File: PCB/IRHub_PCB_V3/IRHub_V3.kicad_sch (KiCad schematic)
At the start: 85 parts, among them Q1 UMH3N, SW1 SW_Push, U1 DRV2605LDGS

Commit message: power pcb done
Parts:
- 5V1, TP9, T_D+1, T_D-1, T_D6, T_D7, T_GND1, T_RX1, T_TX1: footprint TestPoint:TestPoint_Pad_D2.0mm -> TestPoint:TestPoint_Pad_D1.0mm
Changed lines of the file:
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@@
 			)
 		)
-		(property "Footprint" "TestPoint:TestPoint_Pad_D2.0mm"
+		(property "Footprint" "TestPoint:TestPoint_Pad_D1.0mm"
 			(at 267.97 156.21 0)
 			(effects
@@
 			)
 		)
-		(property "Footprint" "TestPoint:TestPoint_Pad_D2.0mm"
+		(property "Footprint" "TestPoint:TestPoint_Pad_D1.0mm"
 			(at 267.97 130.81 0)
 			(effects
@@
 			)
 		)
-		(property "Footprint" "TestPoint:TestPoint_Pad_D2.0mm"
+		(property "Footprint" "TestPoint:TestPoint_Pad_D1.0mm"
 			(at 267.97 149.86 0)
 			(effects
@@
 			)
 		)
-		(property "Footprint" "TestPoint:TestPoint_Pad_D2.0mm"
+		(property "Footprint" "TestPoint:TestPoint_Pad_D1.0mm"
 			(at 267.97 128.27 0)
 			(effects
@@
 			)
 		)
-		(property "Footprint" "TestPoint:TestPoint_Pad_D2.0mm"
+		(property "Footprint" "TestPoint:TestPoint_Pad_D1.0mm"
 			(at 267.97 147.32 0)
 			(effects
@@
 			)
 		)
-		(property "Footprint" "TestPoint:TestPoint_Pad_D2.0mm"
+		(property "Footprint" "TestPoint:TestPoint_Pad_D1.0mm"
 			(at 267.97 166.37 0)
 			(effects
@@
 			)
 		)
-		(property "Footprint" "TestPoint:TestPoint_Pad_D2.0mm"
+		(property "Footprint" "TestPoint:TestPoint_Pad_D1.0mm"
 			(at 267.97 158.75 0)
 			(effects
@@
 			)
 		)
-		(property "Footprint" "TestPoint:TestPoint_Pad_D2.0mm"
+		(property "Footprint" "TestPoint:TestPoint_Pad_D1.0mm"
 			(at 267.97 137.16 0)
 			(effects
@@
 			)
 		)
-		(property "Footprint" "TestPoint:TestPoint_Pad_D2.0mm"
+		(property "Footprint" "TestPoint:TestPoint_Pad_D1.0mm"
 			(at 267.97 139.7 0)
 			(effects

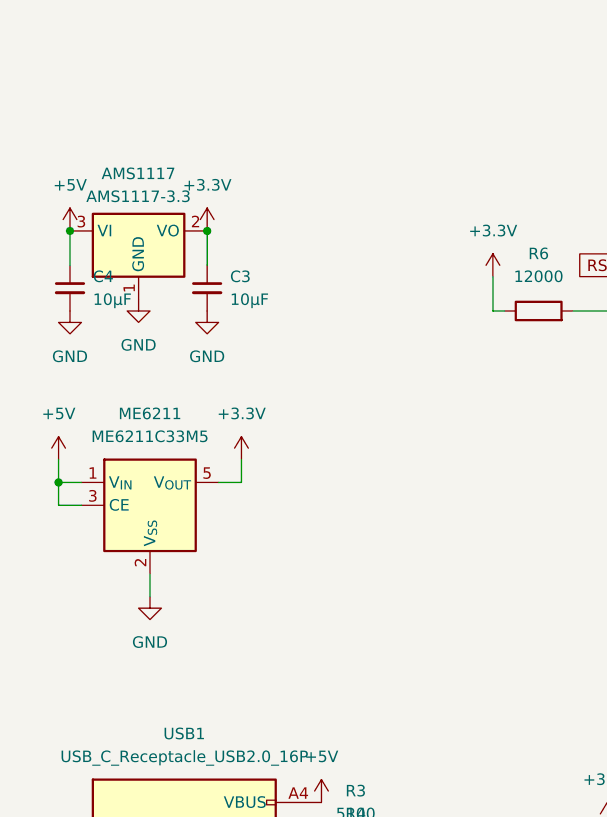
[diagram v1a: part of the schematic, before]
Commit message: finished placement
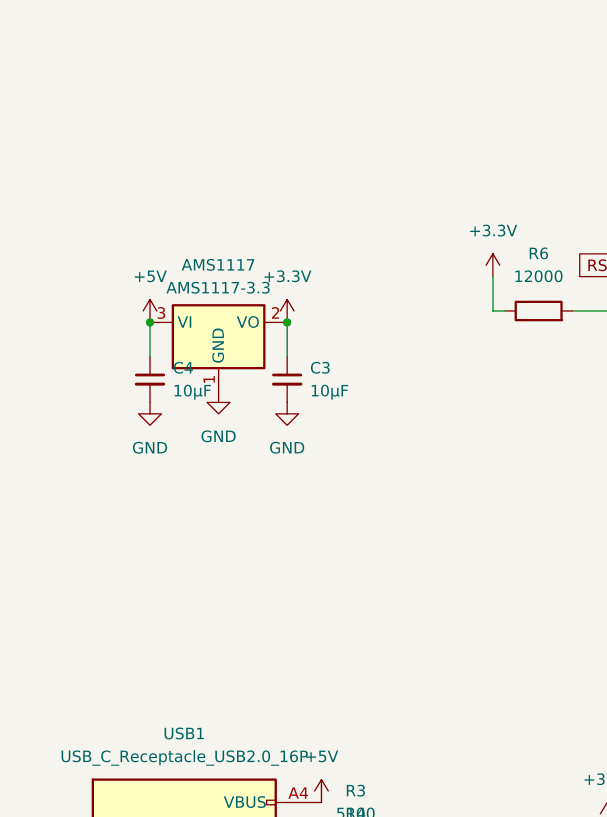
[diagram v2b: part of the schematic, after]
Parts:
- removed ME6211: ME6211C33M5, Package_TO_SOT_SMD:SOT-23-5, symbol Regulator_Linear:ME6211C33M5
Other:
- moved on the sheet: AMS1117, C3, C4
